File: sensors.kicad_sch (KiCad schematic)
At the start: 18 parts, among them IC2 MMC5603NJ, IC3 ICM-42670-P, IC4 MAX-F10S-00B, IC5 ICM-45686, J1 antenna, U2 BMP581

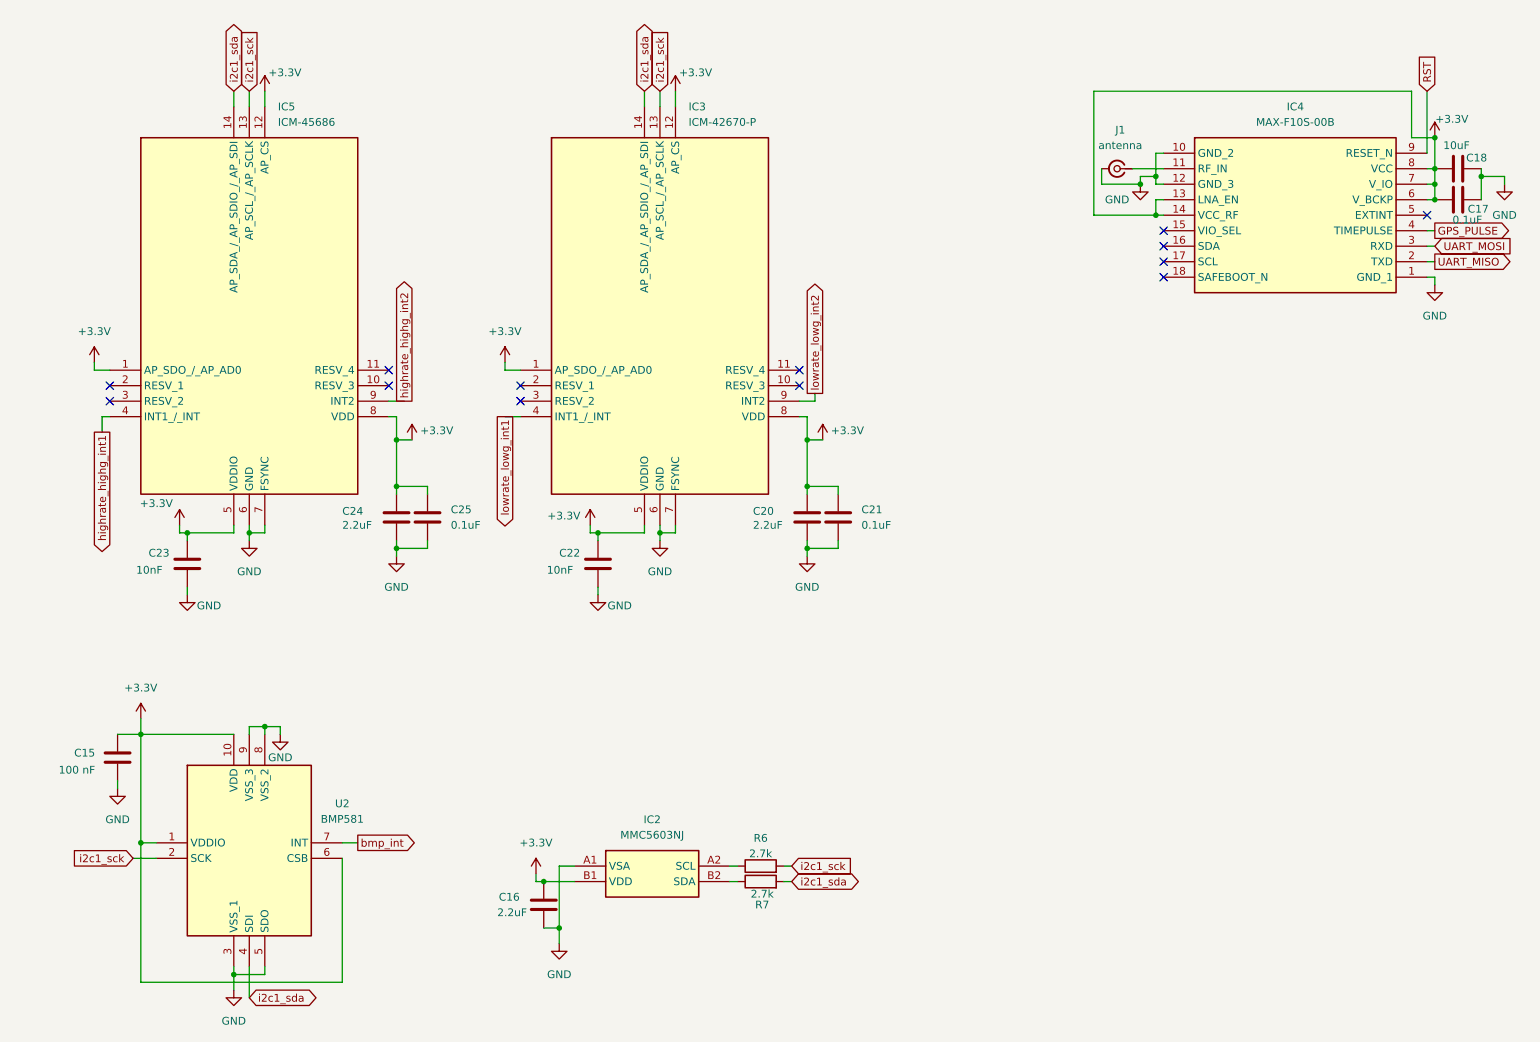
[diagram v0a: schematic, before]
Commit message: tons of work, see journal for details
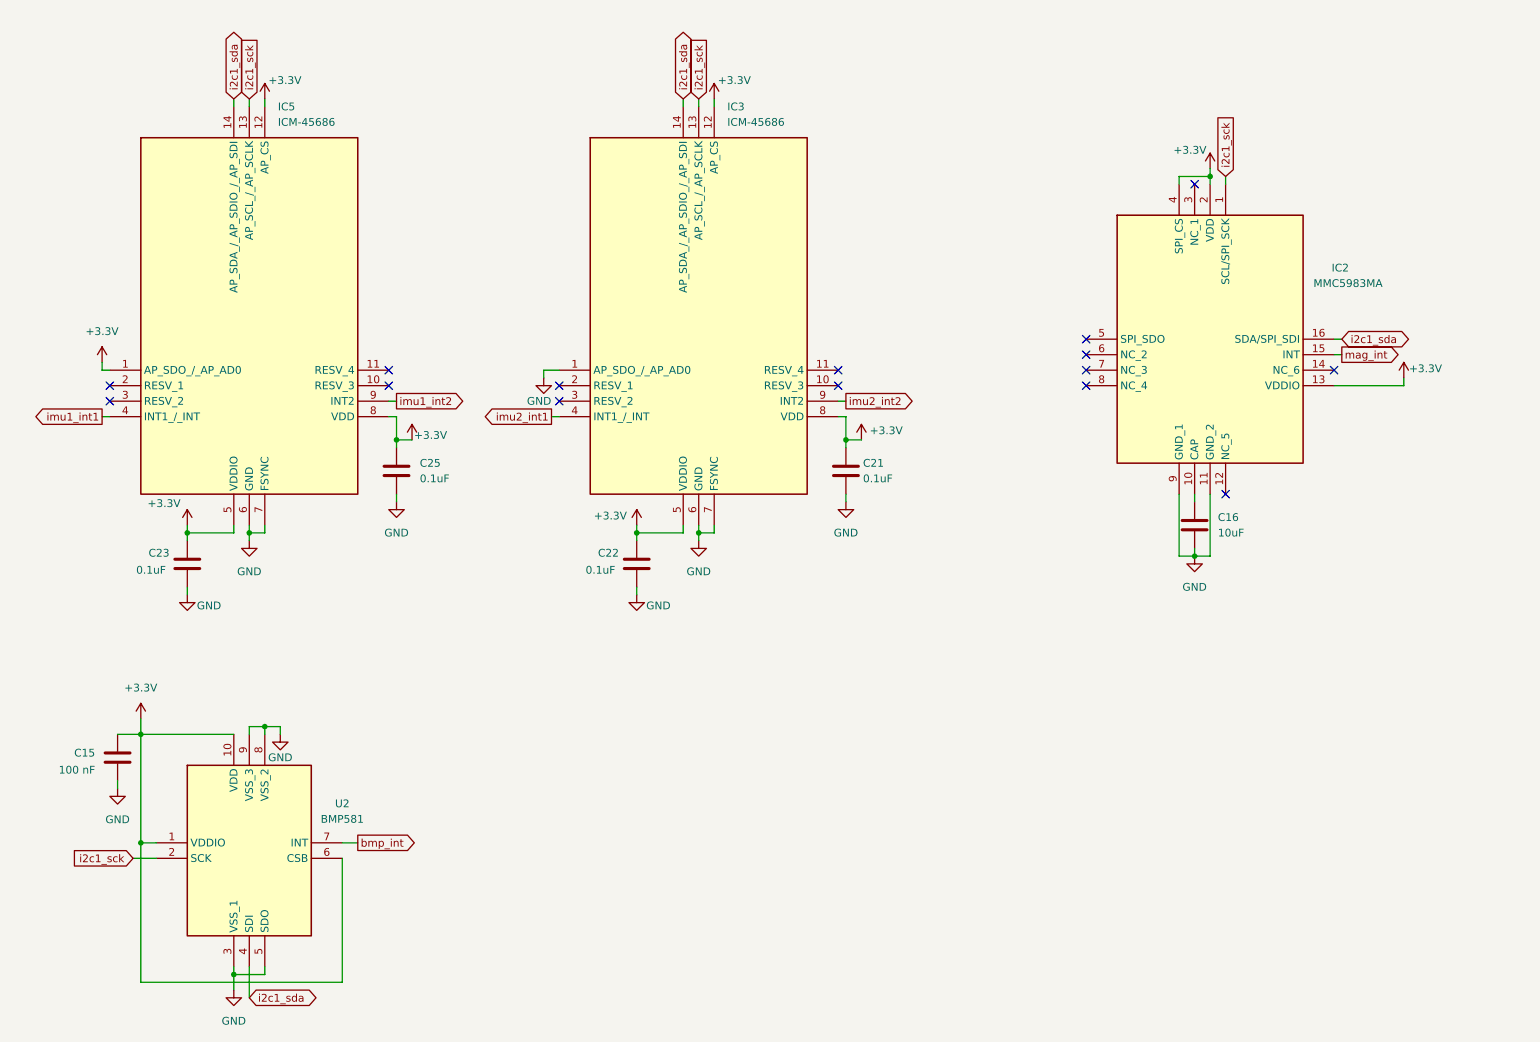
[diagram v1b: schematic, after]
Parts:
- removed C17: 0.1uF, Capacitor_SMD:C_0402_1005Metric, symbol Device:C
- removed C18: 10uF, Capacitor_SMD:C_0603_1608Metric, symbol Device:C
- removed C20, C24: 2.2uF, Capacitor_SMD:C_0603_1608Metric, symbol Device:C
- removed IC2: MMC5603NJ, footprints:MMC5603NJ, symbol MMC5603NJ:MMC5603NJ
- removed IC4: MAX-F10S-00B, footprints:MAXF10S00B, symbol MAX-F10S-00B:MAX-F10S-00B
- removed J1: antenna, Connector_Coaxial:U.FL_Molex_MCRF_73412-0110_Vertical, symbol Connector:Conn_Coaxial_Small
- removed R6, R7: 2.7k, Resistor_SMD:R_0402_1005Metric, symbol Device:R
- added IC2: MMC5983MA, MMC5983MA, symbol MMC5983MA:MMC5983MA
- C16: value 2.2uF -> 10uF; footprint Capacitor_SMD:C_0603_1608Metric -> (none)
- C22, C23: value 10nF -> 0.1uF
- IC3: value ICM-42670-P -> ICM-45686
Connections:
- net +3.3V: now also IC2.13 (VDDIO), IC2.2 (VDD), IC2.4 (SPI_CS); no longer C16.2, IC3.1 (AP_SDO_/_AP_AD0)
- net GND: now also C16.2, IC3.1 (AP_SDO_/_AP_AD0), IC2.11 (GND_2), IC2.9 (GND_1); no longer C16.1
- net i2c1_sck: now also IC2.1 (SCL/SPI_SCK)
- net i2c1_sda: now also IC2.16 (SDA/SPI_SDI)
- net highrate_highg_int1 renamed imu1_int1
- net highrate_highg_int2 renamed imu1_int2
- net lowrate_lowg_int1 renamed imu2_int1
- net lowrate_lowg_int2 renamed imu2_int2
- new net: C16.1, IC2.10 (CAP)
- new net mag_int: IC2.15 (INT)
- no-connect marks 13 -> 15
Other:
- moved on the sheet: C21, C22, C25, IC3
